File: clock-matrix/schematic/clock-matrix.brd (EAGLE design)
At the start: 30 x 50 mm, 85 parts, among them IC1 WS2811-SOP8, IC2 WS2811-SOP8, IC3 74HC595D, U2 ATMEGA328P-MU, X2 USB-MICROB

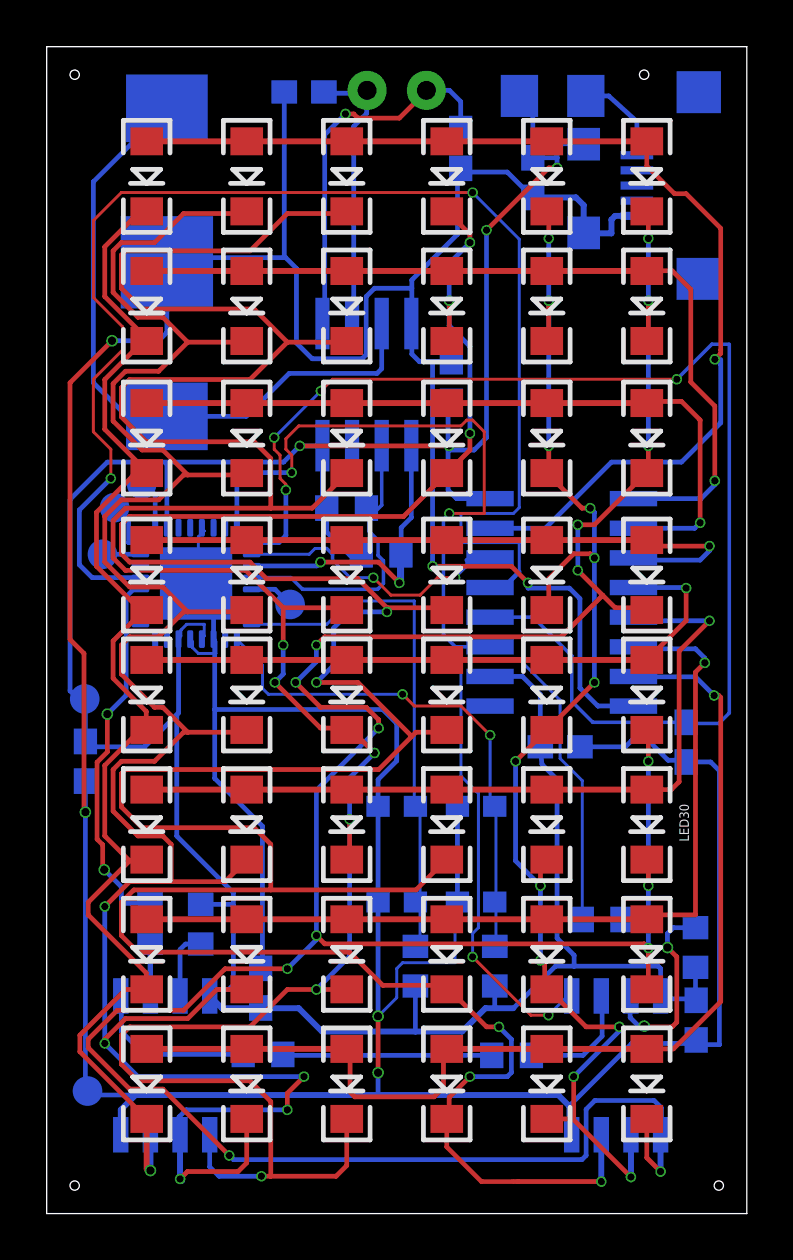
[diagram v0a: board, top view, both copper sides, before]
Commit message: Minor board fixes and other changes
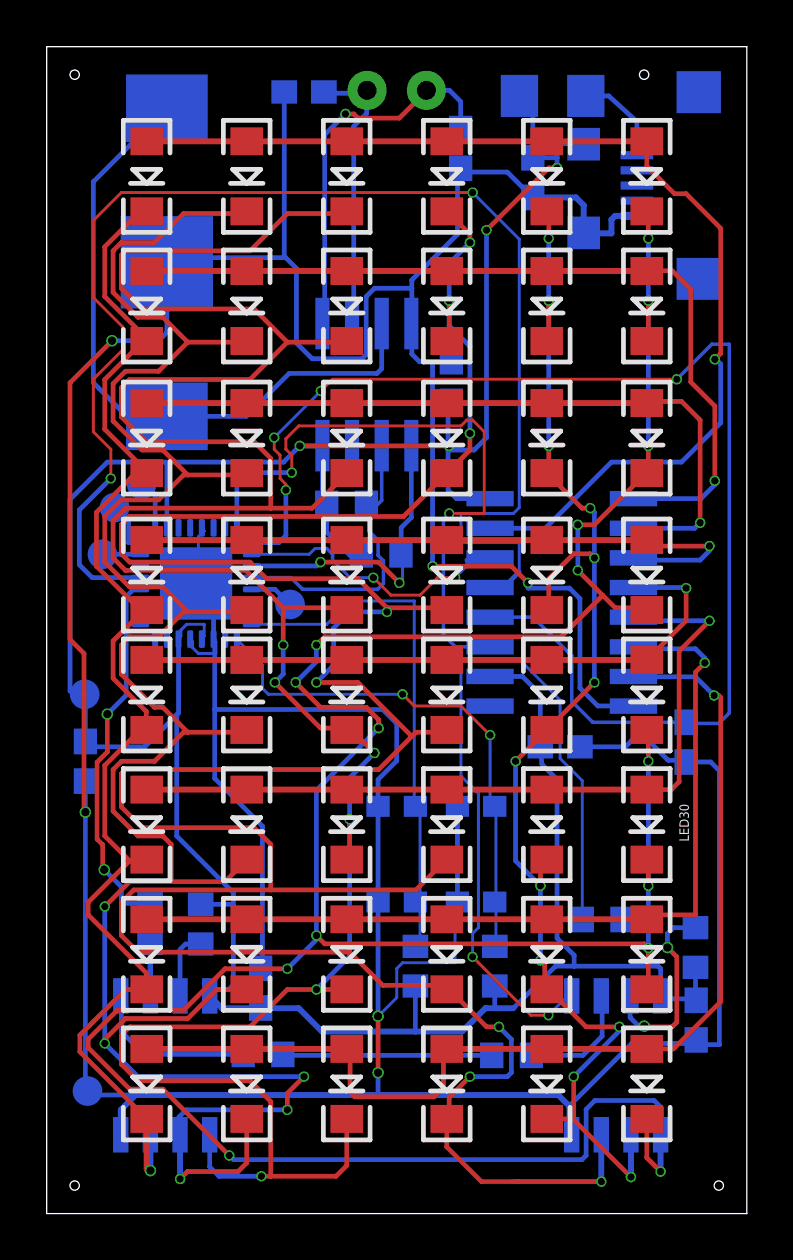
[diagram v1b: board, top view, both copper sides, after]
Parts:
- moved R15 0.20 mm to (12.8, 30.4)
- moved TP6 0.20 mm to (1.63, 22.2)
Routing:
- net SDA: track 14.4 -> 13.3 mm
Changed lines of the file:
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@@
 <drawing>
 <settings>
-<setting alwaysvectorfont="no"/>
+<setting alwaysvectorfont="yes"/>
 <setting verticaltext="up"/>
 </settings>
@@
 </class>
 </classes>
-<designrules name="jlcpcb-2layers">
+<designrules name="jlcpcb-2layers *">
 <description language="en">&lt;b&gt;JLCPCB design rules (2 layers)&lt;/b&gt;
 &lt;ul&gt;
@@
 <param name="mlMinCreamFrame" value="0mil"/>
 <param name="mlMaxCreamFrame" value="0mil"/>
-<param name="mlViaStopLimit" value="0mil"/>
+<param name="mlViaStopLimit" value="14mil"/>
 <param name="srRoundness" value="0"/>
 <param name="srMinRoundness" value="0mil"/>
@@
 <attribute name="NAME" x="12.695" y="27.195" size="1.27" layer="26" rot="MR180"/>
 </element>
-<element name="R15" library="rcl" package="R0603" value="10K" x="12.85" y="30.23" smashed="yes" rot="MR180">
-<attribute name="NAME" x="14.415" y="30.795" size="1.27" layer="26" rot="MR180"/>
+<element name="R15" library="rcl" package="R0603" value="10K" x="12.85" y="30.43" smashed="yes" rot="MR180">
+<attribute name="NAME" x="14.415" y="30.995" size="1.27" layer="26" rot="MR180"/>
 </element>
 <element name="R6" library="adafruit" package="R0603" value="33" x="19.92" y="6.78" smashed="yes" rot="MR180">
@@
 <attribute name="VALUE" x="2.385" y="4.488" size="0.0254" layer="28" rot="MR0"/>
 </element>
-<element name="TP6" library="testpad" package="B1,27" value="TPB1,27" x="1.63" y="22.05" smashed="yes" rot="MR0">
-<attribute name="TP_SIGNAL_NAME" value="" x="2.265" y="20.145" size="1" layer="38" rot="MR0"/>
-<attribute name="VALUE" x="2.265" y="21.288" size="0.0254" layer="28" rot="MR0"/>
-<attribute name="VALUE" x="2.265" y="21.288" size="0.0254" layer="28" rot="MR0"/>
+<element name="TP6" library="testpad" package="B1,27" value="TPB1,27" x="1.63" y="22.25" smashed="yes" rot="MR0">
+<attribute name="TP_SIGNAL_NAME" value="" x="2.265" y="20.345" size="1" layer="38" rot="MR0"/>
+<attribute name="VALUE" x="2.265" y="21.488" size="0.0254" layer="28" rot="MR0"/>
+<attribute name="VALUE" x="2.265" y="21.488" size="0.0254" layer="28" rot="MR0"/>
 </element>
 <element name="U$2" library="SparkFun" package="SO08" value="DS1307SO8" x="13.72" y="35.52" smashed="yes" rot="MR180">
@@
 <wire x1="14.2" y1="18.6" x2="15" y2="19.4" width="0.2032" layer="16"/>
 <wire x1="22.85" y1="22.51589375" x2="23.616075" y2="21.74981875" width="0.2032" layer="16"/>
-<wire x1="23.62089375" y1="21.745" x2="23.616075" y2="21.74981875" width="0.2032" layer="16"/>
 <wire x1="22.85" y1="22.51589375" x2="22.85" y2="26.35" width="0.2032" layer="16"/>
 <wire x1="14.075" y1="13.475" x2="14.2" y2="13.35" width="0.2032" layer="16"/>
@@
 <wire x1="1.6" y1="17.2" x2="1.66" y2="17.2" width="0.2032" layer="1"/>
 <via x="1.66" y="17.2" extent="1-16" drill="0.35"/>
-<wire x1="1.6" y1="17.2" x2="1.6" y2="24" width="0.2032" layer="1"/>
+<wire x1="1.6" y1="17.2" x2="1.6" y2="22.2" width="0.2032" layer="1"/>
+<wire x1="1.6" y1="22.2" x2="1.6" y2="24" width="0.2032" layer="1"/>
 <wire x1="14.2" y1="8.4576" x2="14.2" y2="8.4" width="0.2032" layer="16"/>
 <via x="14.2" y="8.4576" extent="1-16" drill="0.35"/>
@@
 <contactref element="LED13" pad="C"/>
 <wire x1="4.445" y1="3.3766" x2="4.445" y2="1.845" width="0.254" layer="16"/>
-<wire x1="4.445" y1="1.845" x2="4.4" y2="1.8" width="0.254" layer="16"/>
 <wire x1="4.285709375" y1="4.0555" x2="4.285709375" y2="1.914290625" width="0.254" layer="1"/>
 <wire x1="4.285709375" y1="1.914290625" x2="4.4" y2="1.8" width="0.254" layer="1"/>
@@
 <wire x1="14.224" y1="27.9146" x2="11.7348" y2="27.9146" width="0.2032" layer="1"/>
 <wire x1="15.113" y1="27.0256" x2="14.224" y2="27.9146" width="0.2032" layer="1"/>
-<wire x1="15.113" y1="28.0924" x2="15.113" y2="27.0256" width="0.2032" layer="16"/>
 <via x="11.7348" y="27.9146" extent="1-16" drill="0.3048"/>
 <via x="15.113" y="27.0256" extent="1-16" drill="0.3048"/>
@@
 <contactref element="U2" pad="28"/>
 <contactref element="R15" pad="2"/>
-<wire x1="13.75" y1="30" x2="14" y2="30" width="0.127" layer="16"/>
+<wire x1="13.793478125" y1="30" x2="13.8" y2="30" width="0.127" layer="16"/>
+<wire x1="13.8" y1="30" x2="14" y2="30" width="0.127" layer="16"/>
 <wire x1="14" y1="30" x2="14.0472" y2="30.0472" width="0.127" layer="16"/>
-<wire x1="13.75" y1="30" x2="13.7" y2="30.23" width="0.127" layer="16"/>
+<wire x1="13.793478125" y1="30" x2="13.7" y2="30.43" width="0.127" layer="16"/>
 <wire x1="8.8" y1="27.25" x2="8.785" y2="27.25" width="0.127" layer="16"/>
 <wire x1="14.25" y1="32.75" x2="14.355" y2="32.9038" width="0.127" layer="16"/>
-<wire x1="14.355" y1="32.9038" x2="14.355" y2="30.355" width="0.1524" layer="16"/>
-<wire x1="14.355" y1="30.355" x2="14" y2="30" width="0.1524" layer="16"/>
-<wire x1="13.7" y1="30.23" x2="13.8" y2="30.13" width="0.1524" layer="16"/>
+<wire x1="14.355" y1="32.9038" x2="14.355" y2="30.555" width="0.1524" layer="16"/>
+<wire x1="14.355" y1="30.555" x2="13.8" y2="30" width="0.1524" layer="16"/>
+<wire x1="13.7" y1="30.43" x2="13.8" y2="30.33" width="0.1524" layer="16"/>
 <wire x1="14.2" y1="28.2" x2="14.2" y2="28.84736875" width="0.1524" layer="16"/>
 <wire x1="13.8" y1="29.24736875" x2="14.2" y2="28.84736875" width="0.1524" layer="16"/>
-<wire x1="13.8" y1="30.13" x2="13.8" y2="29.24736875" width="0.1524" layer="16"/>
+<wire x1="13.8" y1="30.33" x2="13.8" y2="29.24736875" width="0.1524" layer="16"/>
 <wire x1="14.4294" y1="27.9706" x2="14.4294" y2="27" width="0.1524" layer="16"/>
 <wire x1="14.4294" y1="27.9706" x2="14.2" y2="28.2" width="0.1524" layer="16"/>
@@
 <wire x1="19.2" y1="8.8" x2="20" y2="8.8" width="0.254" layer="16"/>
 <wire x1="26.305" y1="9.3234" x2="26.305" y2="9.2" width="0.254" layer="16"/>
-<wire x1="12" y1="29.2" x2="12" y2="30.23" width="0.2032" layer="16"/>
+<wire x1="12" y1="29.2" x2="12" y2="30.43" width="0.2032" layer="16"/>
 <wire x1="12" y1="29.2" x2="13" y2="28.2" width="0.2032" layer="16"/>
 <wire x1="13" y1="28.2" x2="13.45" y2="28.2" width="0.2032" layer="16"/>
 <wire x1="13.45" y1="28.2" x2="13.48" y2="28.23" width="0.2032" layer="16"/>
-<wire x1="11.815" y1="32.9038" x2="11.815" y2="30.415" width="0.2032" layer="16"/>
-<wire x1="11.815" y1="30.415" x2="12" y2="30.23" width="0.2032" layer="16"/>
+<wire x1="11.815" y1="32.9038" x2="11.815" y2="30.615" width="0.2032" layer="16"/>
+<wire x1="11.815" y1="30.615" x2="12" y2="30.43" width="0.2032" layer="16"/>
 <contactref element="IC3" pad="16"/>
 <contactref element="IC3" pad="10"/>
@@
 <wire x1="9.2456" y1="8.89" x2="9.17" y2="8.81" width="0.2032" layer="16"/>
 <wire x1="9.2456" y1="8.89" x2="9.2456" y2="8.8" width="0.2032" layer="16"/>
-<wire x1="21.8694" y1="18.6024" x2="21.8694" y2="14.4" width="0.2032" layer="16"/>
-<wire x1="21.8694" y1="14.4" x2="21.8694" y2="11.8" width="0.2032" layer="16"/>
+<wire x1="21.8694" y1="18.6024" x2="21.8694" y2="11.8" width="0.2032" layer="16"/>
 <wire x1="21.2211125" y1="19.2506875" x2="21.8694" y2="18.6024" width="0.2032" layer="16"/>
 <wire x1="21.2211125" y1="19.2506875" x2="21.150446875" y2="19.995296875" width="0.2032" layer="16"/>
@@
 <wire x1="5.15" y1="32.1" x2="5.25" y2="32.2" width="0.2032" layer="16"/>
 <wire x1="5.65" y1="24.615" x2="5.65" y2="21.45" width="0.2032" layer="16"/>
-<wire x1="5.575" y1="21.375" x2="5.5" y2="21.3" width="0.2032" layer="16"/>
-<wire x1="5.5" y1="21.3" x2="4.2" y2="20" width="0.2032" layer="16"/>
+<wire x1="5.575" y1="21.375" x2="4.2" y2="20" width="0.2032" layer="16"/>
 <wire x1="1.88655625" y1="20" x2="4.2" y2="20" width="0.2032" layer="16"/>
 <wire x1="1.88655625" y1="20" x2="1.6622125" y2="20.22434375" width="0.2032" layer="16"/>
 <wire x1="1.88655625" y1="20" x2="1.84524375" y2="20" width="0.2032" layer="16"/>
 <wire x1="1.84524375" y1="20" x2="1.68876875" y2="20.156475" width="0.2032" layer="16"/>
-<wire x1="1.66" y1="22.02" x2="1.66" y2="20.23" width="0.2032" layer="16"/>
+<wire x1="1.66" y1="22.02" x2="1.66" y2="21.8" width="0.2032" layer="16"/>
+<wire x1="1.66" y1="21.8" x2="1.66" y2="20.23" width="0.2032" layer="16"/>
 <wire x1="6.985" y1="9.6" x2="6.985" y2="9.3234" width="0.2032" layer="16"/>
 <wire x1="5.575" y1="21.375" x2="5.575" y2="16.175" width="0.2032" layer="16"/>
 <wire x1="5.575" y1="21.375" x2="5.65" y2="21.45" width="0.2032" layer="16"/>
 <wire x1="1" y1="30.6" x2="1" y2="22.4" width="0.2032" layer="16"/>
-<wire x1="1" y1="22.4" x2="1.35" y2="22.05" width="0.2032" layer="16"/>
-<wire x1="1.35" y1="22.05" x2="1.63" y2="22.05" width="0.2032" layer="16"/>
+<wire x1="1" y1="22.4" x2="1.15" y2="22.25" width="0.2032" layer="16"/>
+<wire x1="1.15" y1="22.25" x2="1.63" y2="22.25" width="0.2032" layer="16"/>
 <contactref element="R7" pad="1"/>
 <contactref element="R8" pad="1"/>
@@
 <wire x1="27.8" y1="10.55" x2="27.8" y2="9.23" width="0.2032" layer="16"/>
 <wire x1="27.8" y1="9.23" x2="27.77" y2="9.2" width="0.2032" layer="16"/>
-<wire x1="1.66" y1="22.02" x2="1.63" y2="22.05" width="0" layer="19" extent="16-16"/>
+<wire x1="1.63" y1="22.25" x2="1.66" y2="22.22" width="0.1524" layer="16"/>
+<wire x1="1.66" y1="22.22" x2="1.66" y2="21.8" width="0.1524" layer="16"/>
 </signal>
 <signal name="SER">
@@
 <wire x1="24.2" y1="32.2" x2="27.2" y2="32.2" width="0.2032" layer="16"/>
 <wire x1="28.8824" y1="33.8824" x2="28.8824" y2="36.4" width="0.2032" layer="16"/>
-<wire x1="28.8824" y1="36.4" x2="28.8824" y2="36.6" width="0.2032" layer="16"/>
 <wire x1="27.2" y1="32.2" x2="28.8824" y2="33.8824" width="0.2032" layer="16"/>
 <wire x1="28.8824" y1="36.4" x2="28.6824" y2="36.6" width="0.2032" layer="16"/>
@@
 <wire x1="25.714259375" y1="44.885740625" x2="26.9" y2="43.7" width="0.2" layer="1"/>
 <wire x1="27.4" y1="43.7" x2="28.8824" y2="42.2176" width="0.2" layer="1"/>
-<wire x1="28.8824" y1="42.2176" x2="28.8824" y2="37" width="0.2" layer="1"/>
-<wire x1="28.8824" y1="37" x2="28.8824" y2="36.854" width="0.2" layer="1"/>
+<wire x1="28.8824" y1="42.2176" x2="28.8824" y2="36.854" width="0.2" layer="1"/>
 <wire x1="28.8824" y1="36.854" x2="28.6284" y2="36.6" width="0.2" layer="1"/>
 </signal>
